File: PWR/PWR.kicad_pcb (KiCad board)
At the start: 2 copper layers, 70.1 x 65 mm, 21 parts, among them J1 +12v, P1 +5v, P2 GND, SW1 SPDT

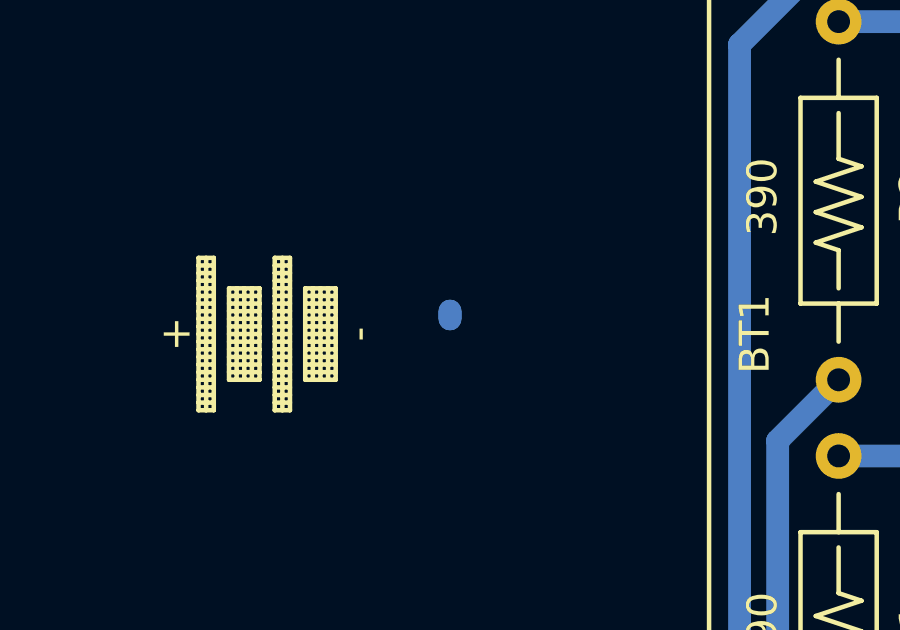
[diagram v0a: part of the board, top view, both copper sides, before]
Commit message: Cleanup...
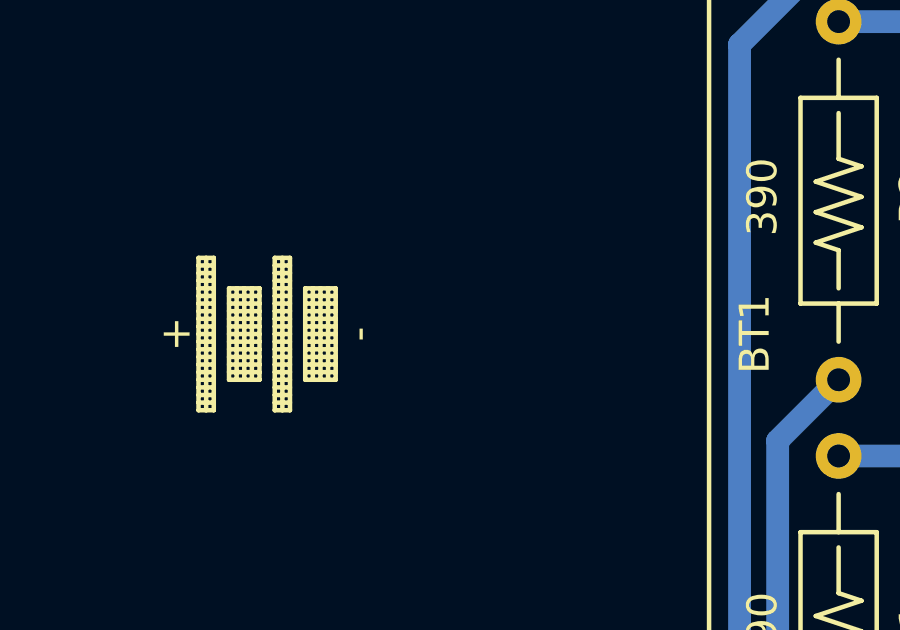
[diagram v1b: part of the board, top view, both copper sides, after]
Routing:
- net (no net): track 0.51 -> 0.00 mm
